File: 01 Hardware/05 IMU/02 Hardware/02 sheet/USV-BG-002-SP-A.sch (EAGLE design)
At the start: 2 parts, among them J2 690367291276, U1 RASPBERRY_PICOTH

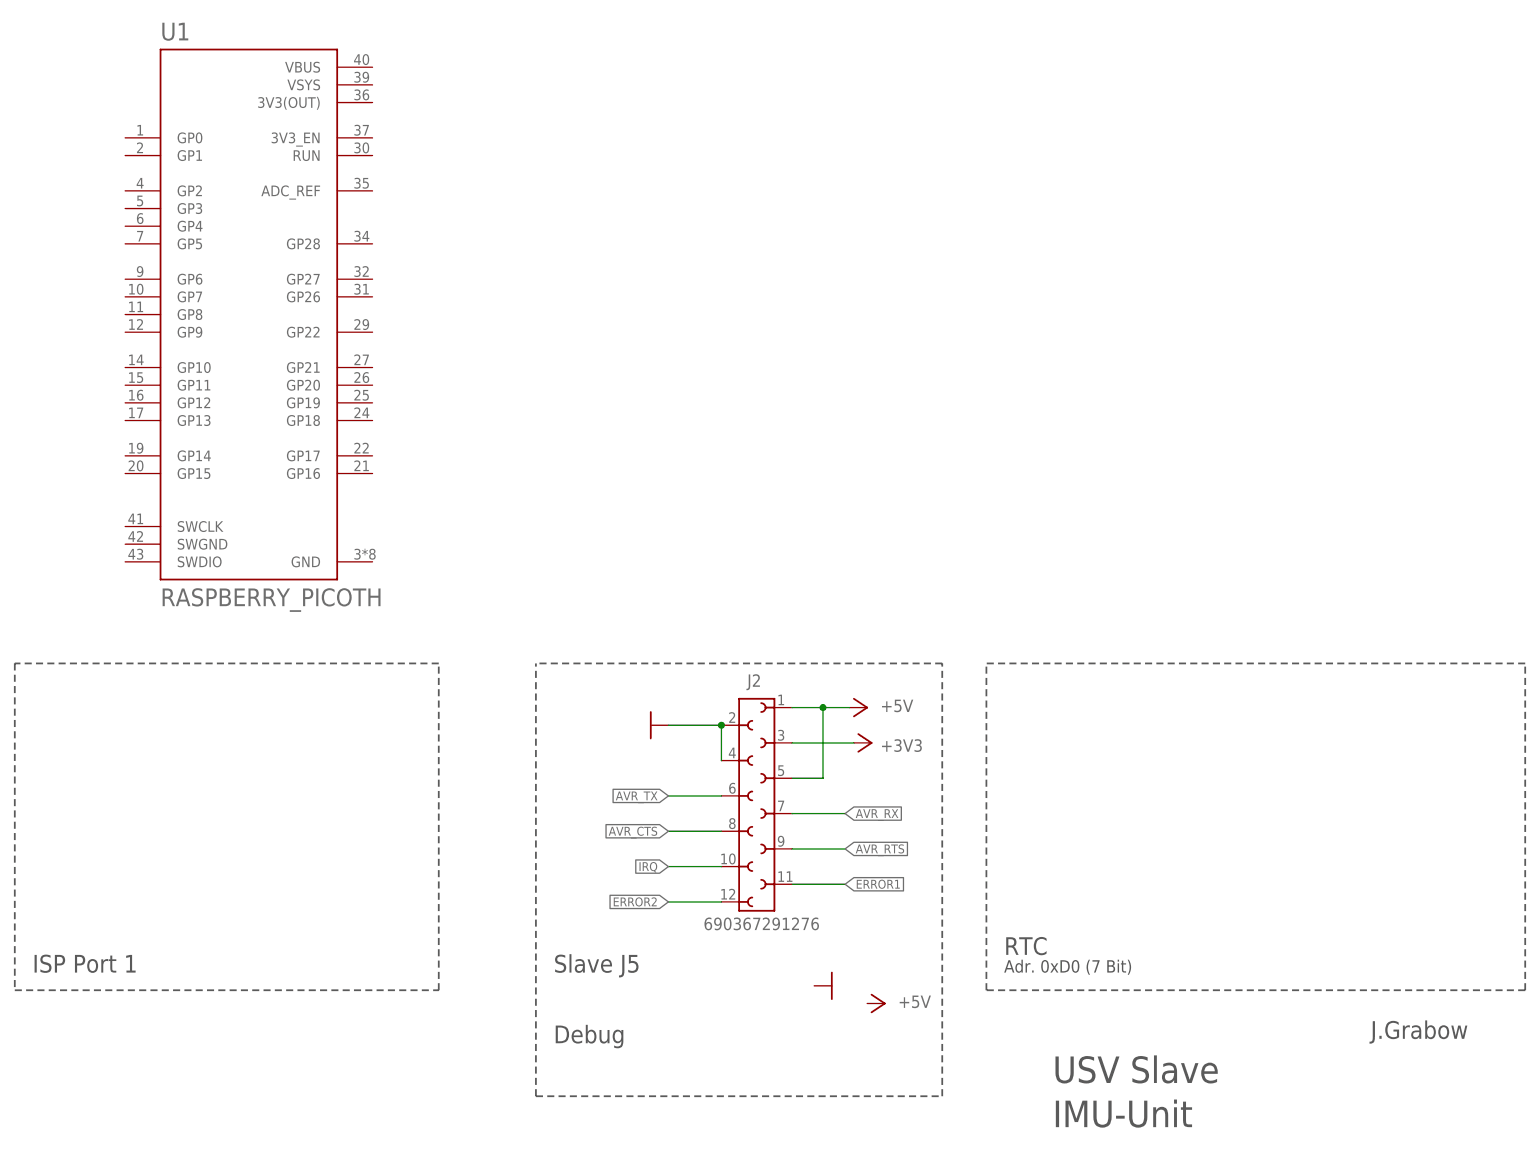
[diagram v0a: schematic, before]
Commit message: Sheet and Board for IMU
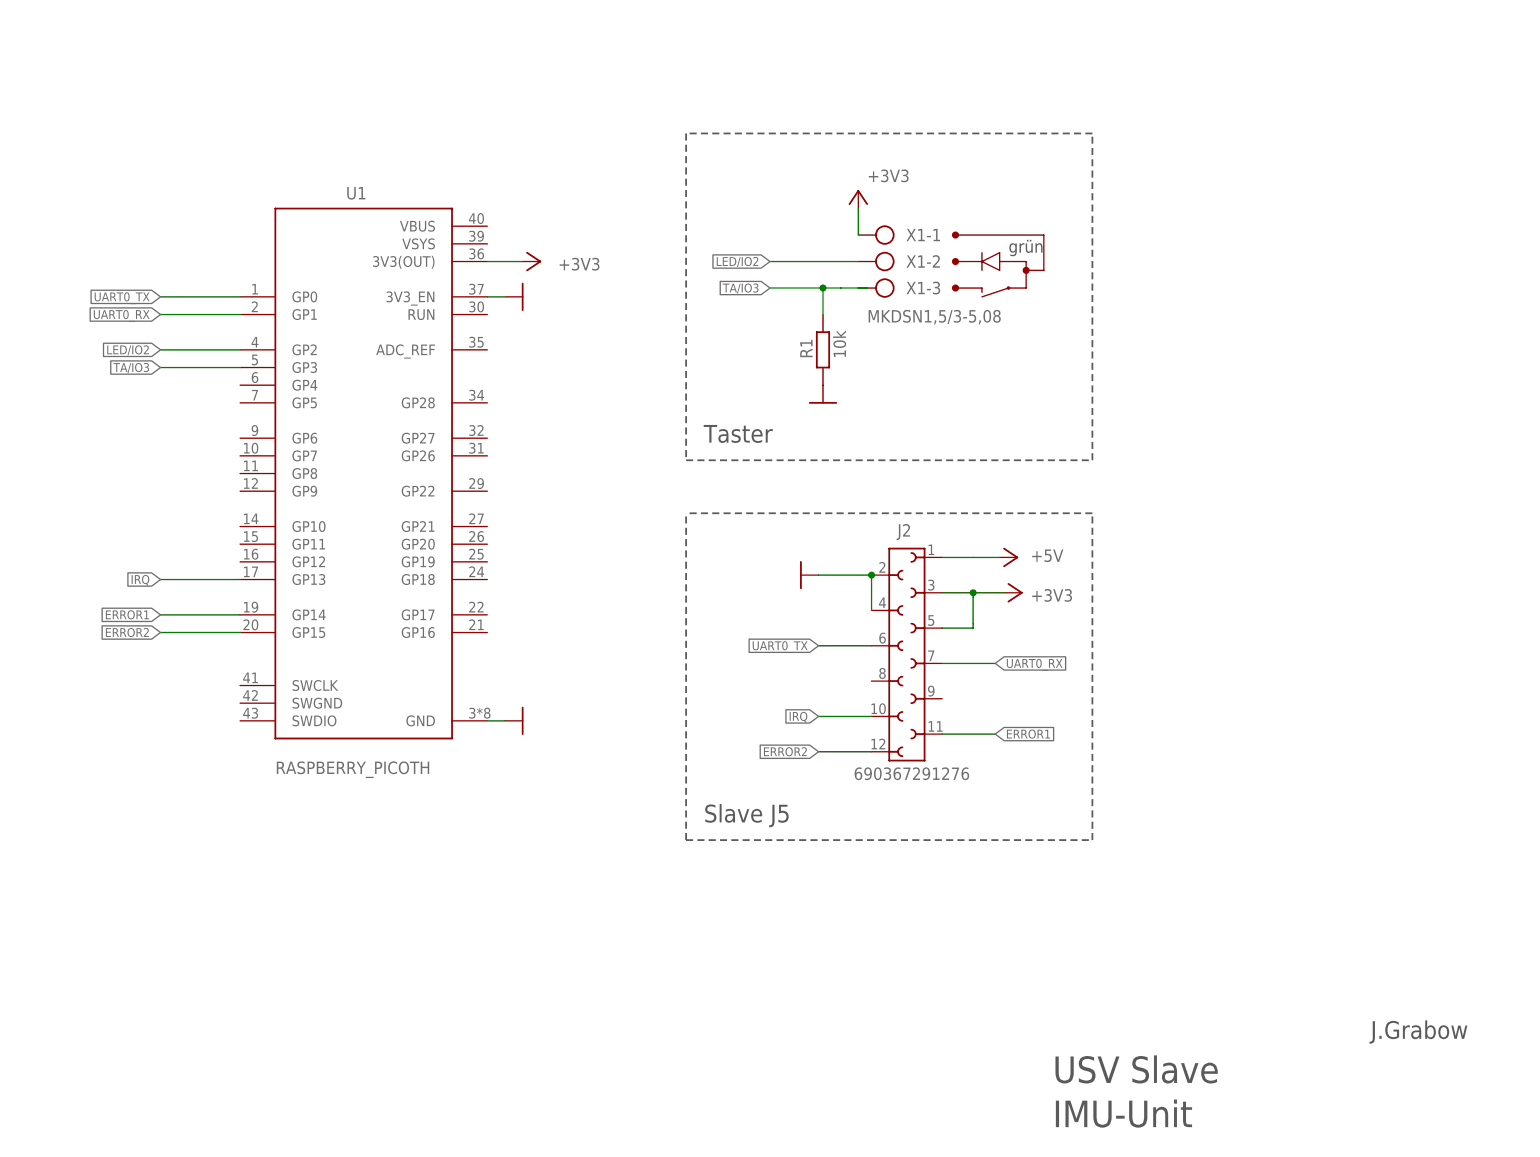
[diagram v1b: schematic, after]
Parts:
- added R1: 10k, rcl:R-EU_M0805
- added X1: MKDSN1,5/3-5,08, con-phoenix-508:MKDSN1,5/3-5,08
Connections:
- removed net AVR_CTS: J2.8
- removed net AVR_RTS: J2.9
- removed net AVR_RX: J2.7
- removed net AVR_TX: J2.6
- new net LED/IO2: U1.GP2, X1-2.KL
- new net TA/IO3: R1.2, U1.GP3, X1-3.KL
- new net UART0_RX: J2.7, U1.GP1
- new net UART0_TX: J2.6, U1.GP0
- net +3V3: now also J2.5, U1.3V3(OUT), X1-1.KL
- net +5V: no longer J2.5
- net ERROR1: now also U1.GP14
- net ERROR2: now also U1.GP15
- net GND: now also R1.1, U1.3V3_EN, U1.GND
- net IRQ: now also U1.GP13
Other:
- note added: "Taster"
- note added: "grün"
- note removed: "Adr. 0xD0 (7 Bit)"
- note removed: "Debug"
- note removed: "ISP Port 1"
- note removed: "RTC"
- moved on the sheet: J2, U1
